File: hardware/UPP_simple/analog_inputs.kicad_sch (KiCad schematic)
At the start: 103 parts, among them J1 Conn_01x03, J10 Conn_01x03, J11 Conn_01x03, J12 Conn_01x03, J13 Conn_01x03, J14 Conn_01x03, J15 Conn_01x03, J16 Conn_01x03, J17 Conn_01x03, J18 Conn_01x03, J19 Conn_01x04, J2 Conn_01x03, J20 Conn_01x03, J21 Conn_01x03, J22 Conn_01x04, J23 Conn_01x03, J24 Conn_01x03, J25 Conn_01x04, J26 Conn_01x03, J27 Conn_01x03, J28 Conn_01x04, J29 Conn_01x04, J3 Conn_01x03, J30 Conn_01x04, J31 Conn_01x03, J32 Conn_01x03, J33 Conn_01x03, J34 Conn_01x03, J35 Conn_01x03, J36 Conn_01x03, J4 Conn_01x03, J5 Conn_01x03, J6 Conn_01x03, J7 Conn_01x03, J8 Conn_01x03, J9 Conn_01x03, U1 Opamp_Quad, U2 Opamp_Quad, U3 Opamp_Quad, U4 Opamp_Quad, U5 Opamp_Quad, U8 Opamp_Quad, U9 Opamp_Quad

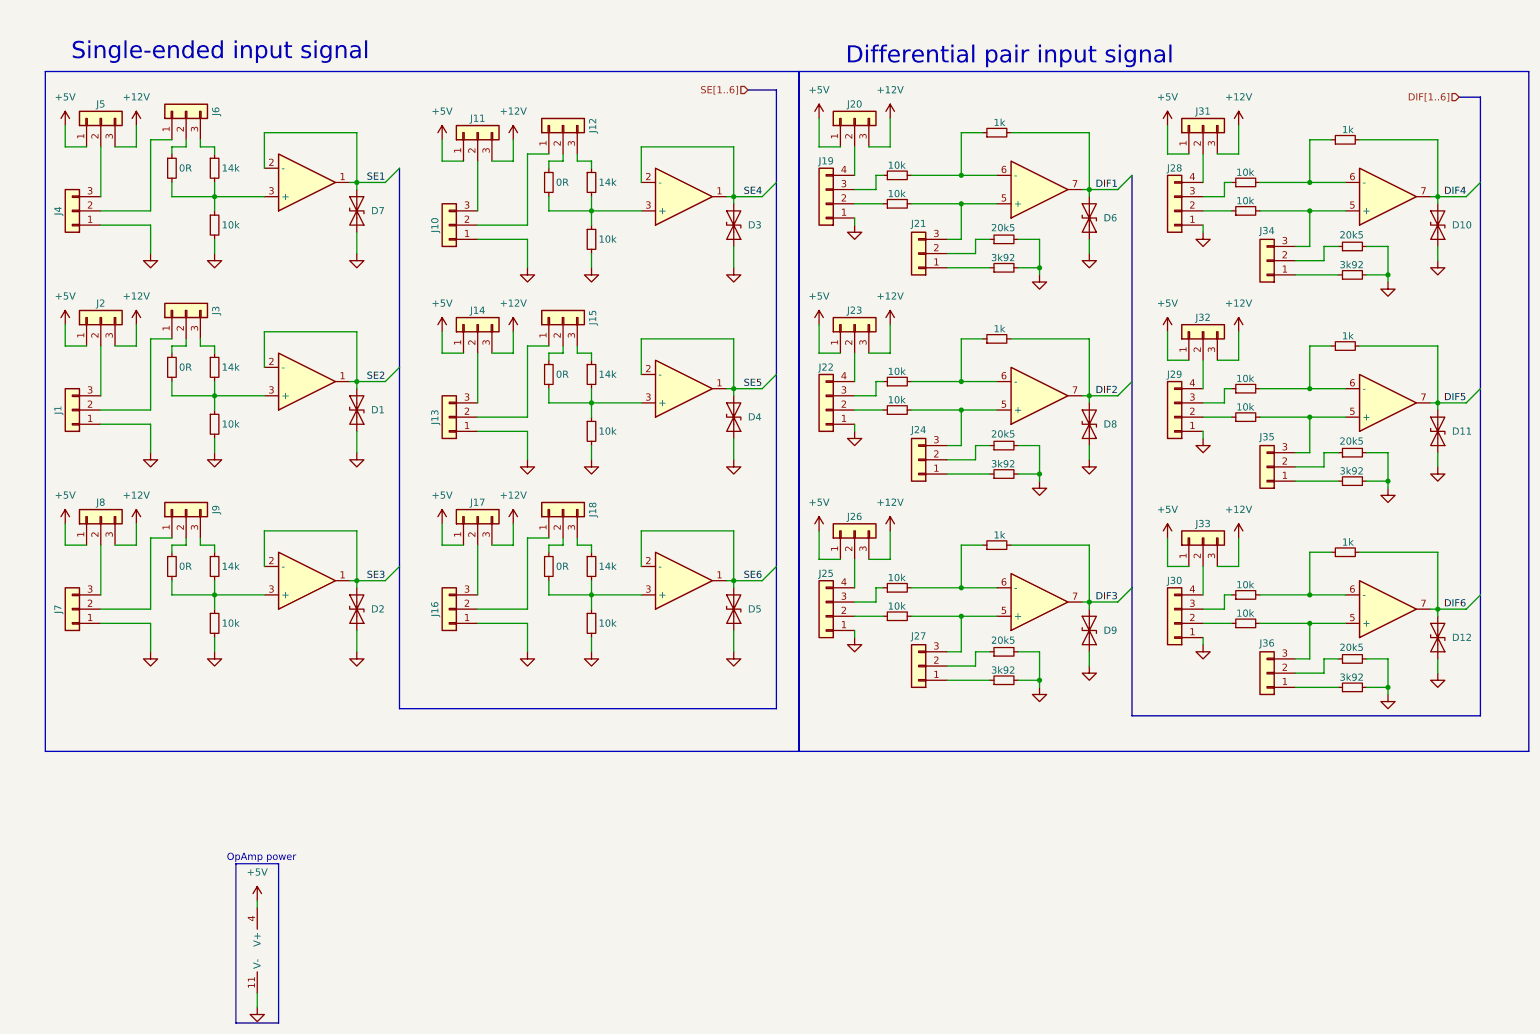
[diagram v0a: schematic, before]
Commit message: Add files via upload
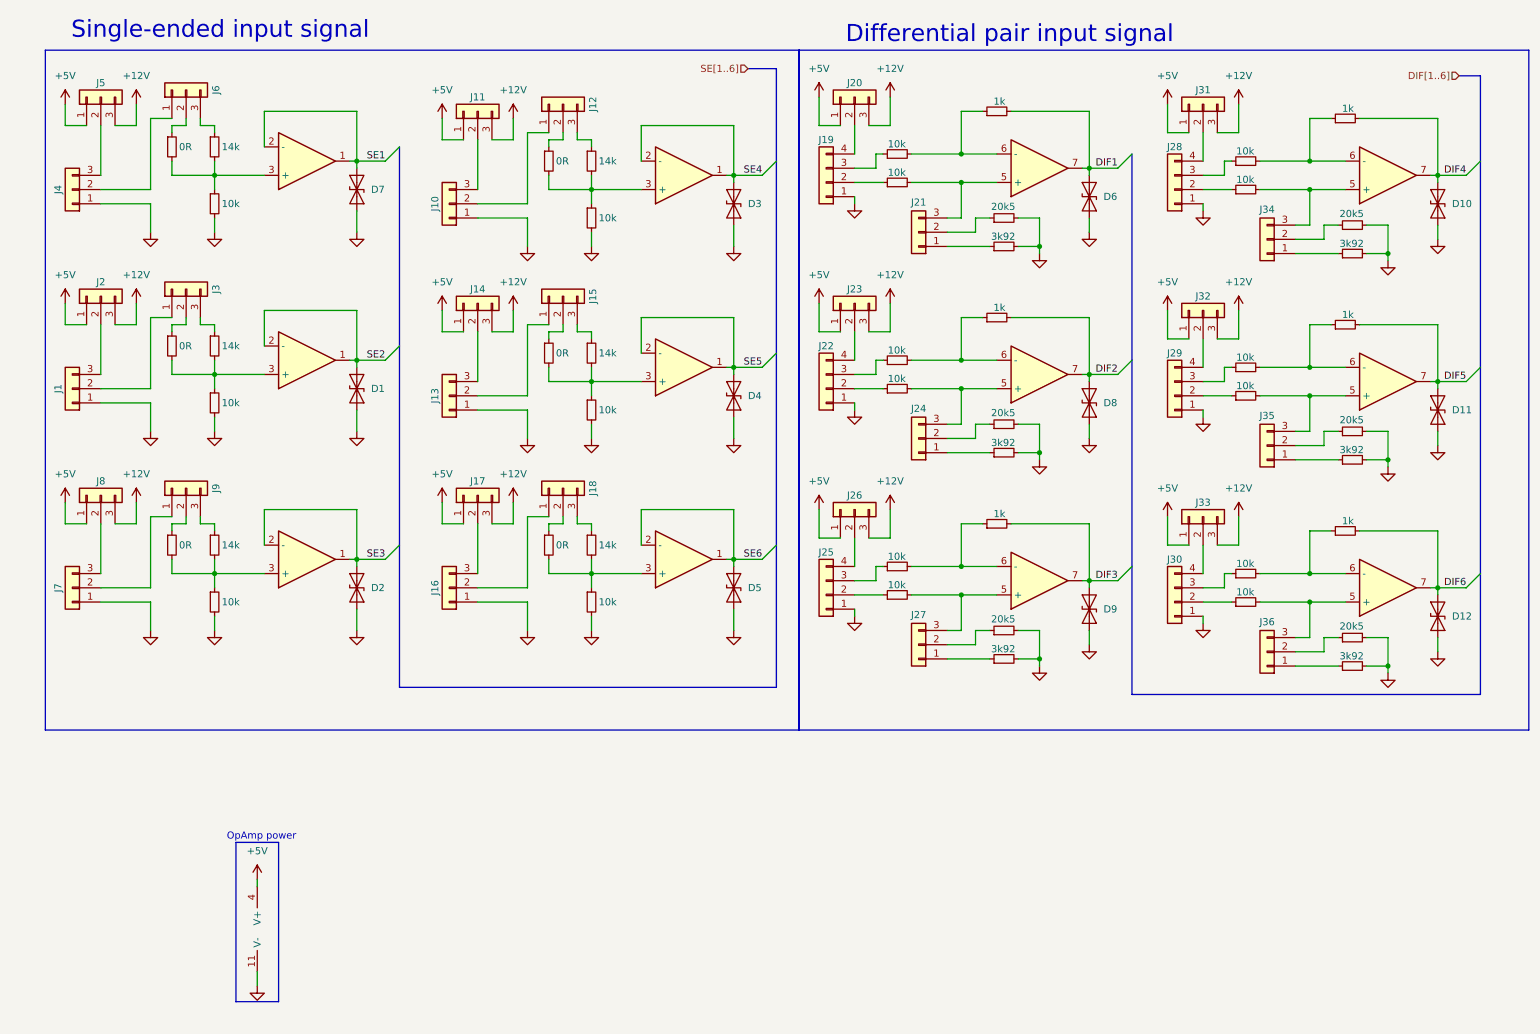
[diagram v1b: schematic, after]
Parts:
- removed R1, R4: 0R, Resistor_SMD:R_0603_1608Metric, symbol Device:R_Small
- removed R2, R5, R6: 14k, Resistor_SMD:R_0603_1608Metric, symbol Device:R_Small
- removed R3, R7: 10k, Resistor_SMD:R_0603_1608Metric, symbol Device:R_Small
- added R16, R8: 0R, Resistor_SMD:R_0603_1608Metric, symbol Device:R_Small
- added R17, R19, R21: 14k, Resistor_SMD:R_0603_1608Metric, symbol Device:R_Small
- added R18, R20: 10k, Resistor_SMD:R_0603_1608Metric, symbol Device:R_Small
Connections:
- net GND: now also R18.2, R20.2
- net at R33.2, U9.3 (+): now also R17.2, R18.1
- net at J3.3 (Pin_3): now also R19.1
- net at U1.3 (+): now also R19.2, R20.1, R8.2
- net at J9.3 (Pin_3): now also R21.1
- net at R16.1, U2.3 (+): now also R16.2, R21.2
- net at J9.2 (Pin_2): now also R16.1
- net at J3.2 (Pin_2): now also R8.1
- net at J6.3 (Pin_3): now also R17.1
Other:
- company: (none) -> Author: Kacper Pawlak
- title: (none) -> Universal use measuring PCB
- moved on the sheet: D1, D10, D11, D12, D2, D3, D4, D5, D6, D7, D8, D9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
